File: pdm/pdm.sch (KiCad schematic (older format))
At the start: 46 parts, among them J1 Conn_01x04_Male, J2 Conn_01x06_Female, J3 Conn_01x04_Female, J4 Conn_01x12_Male, M1 Fan, M2 Fan, SW1 SW_Push, U1 SN65HVD233, U2 STM32F042G6Ux, Y1 Crystal_GND24

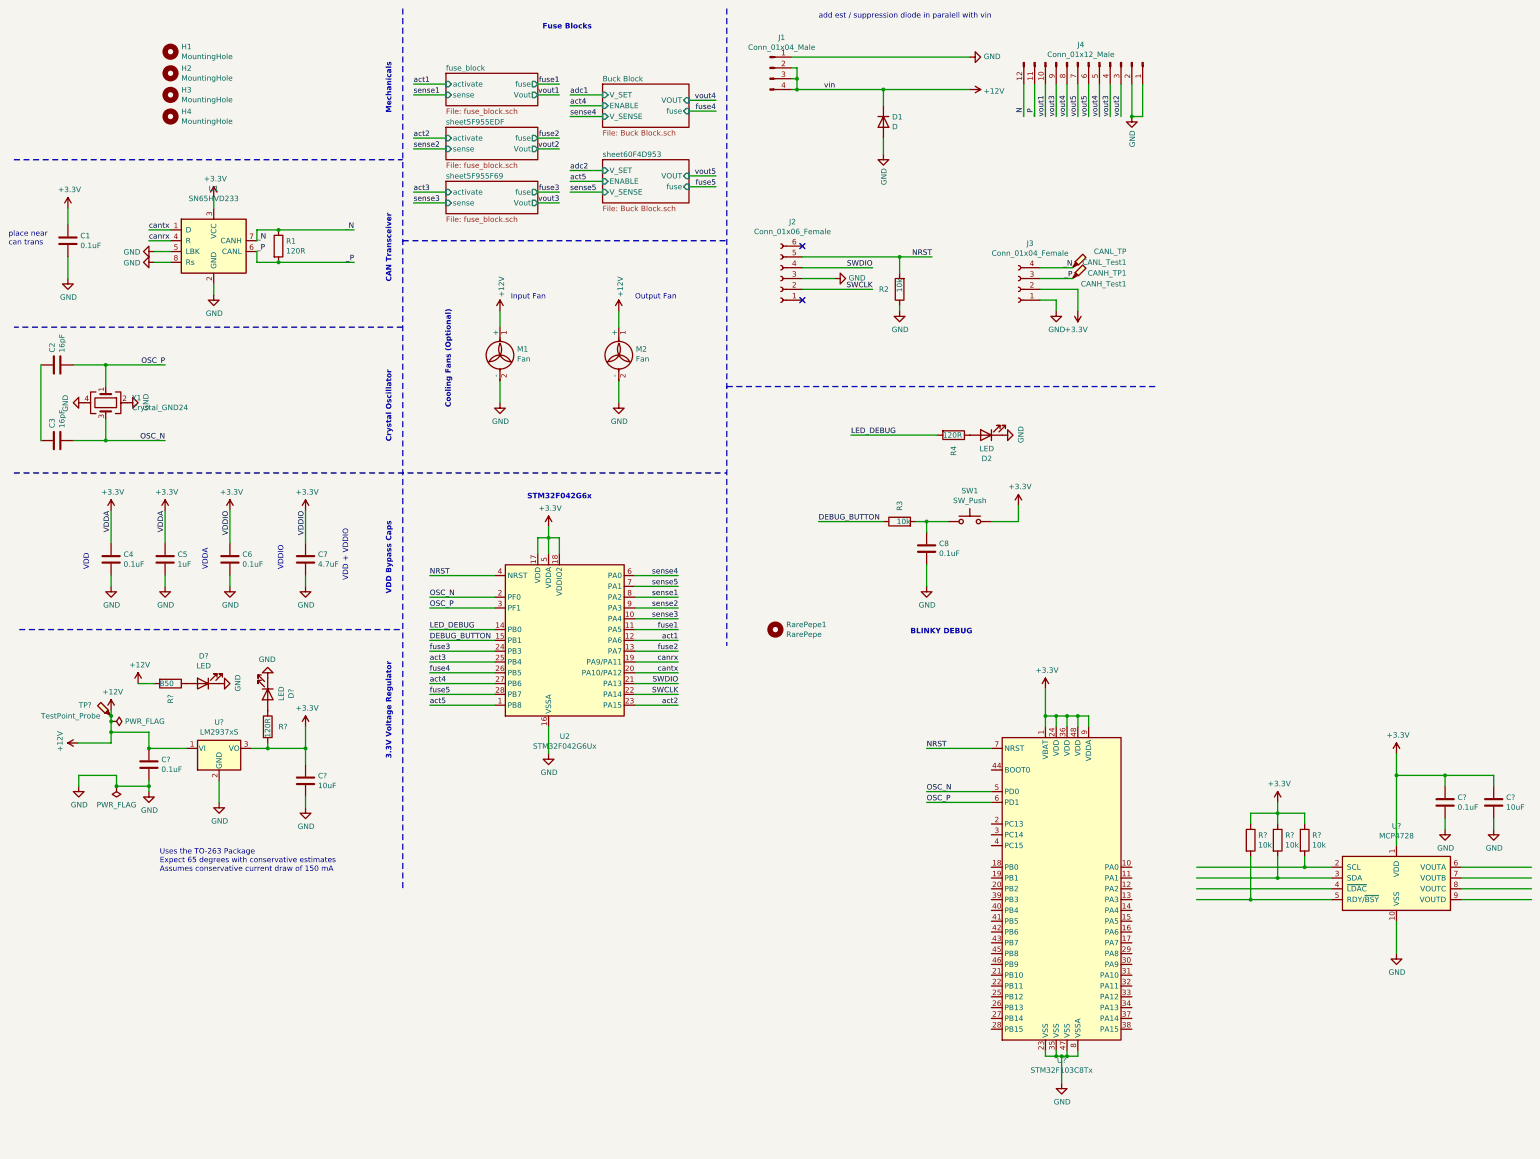
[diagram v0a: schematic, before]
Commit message: fixed schematic
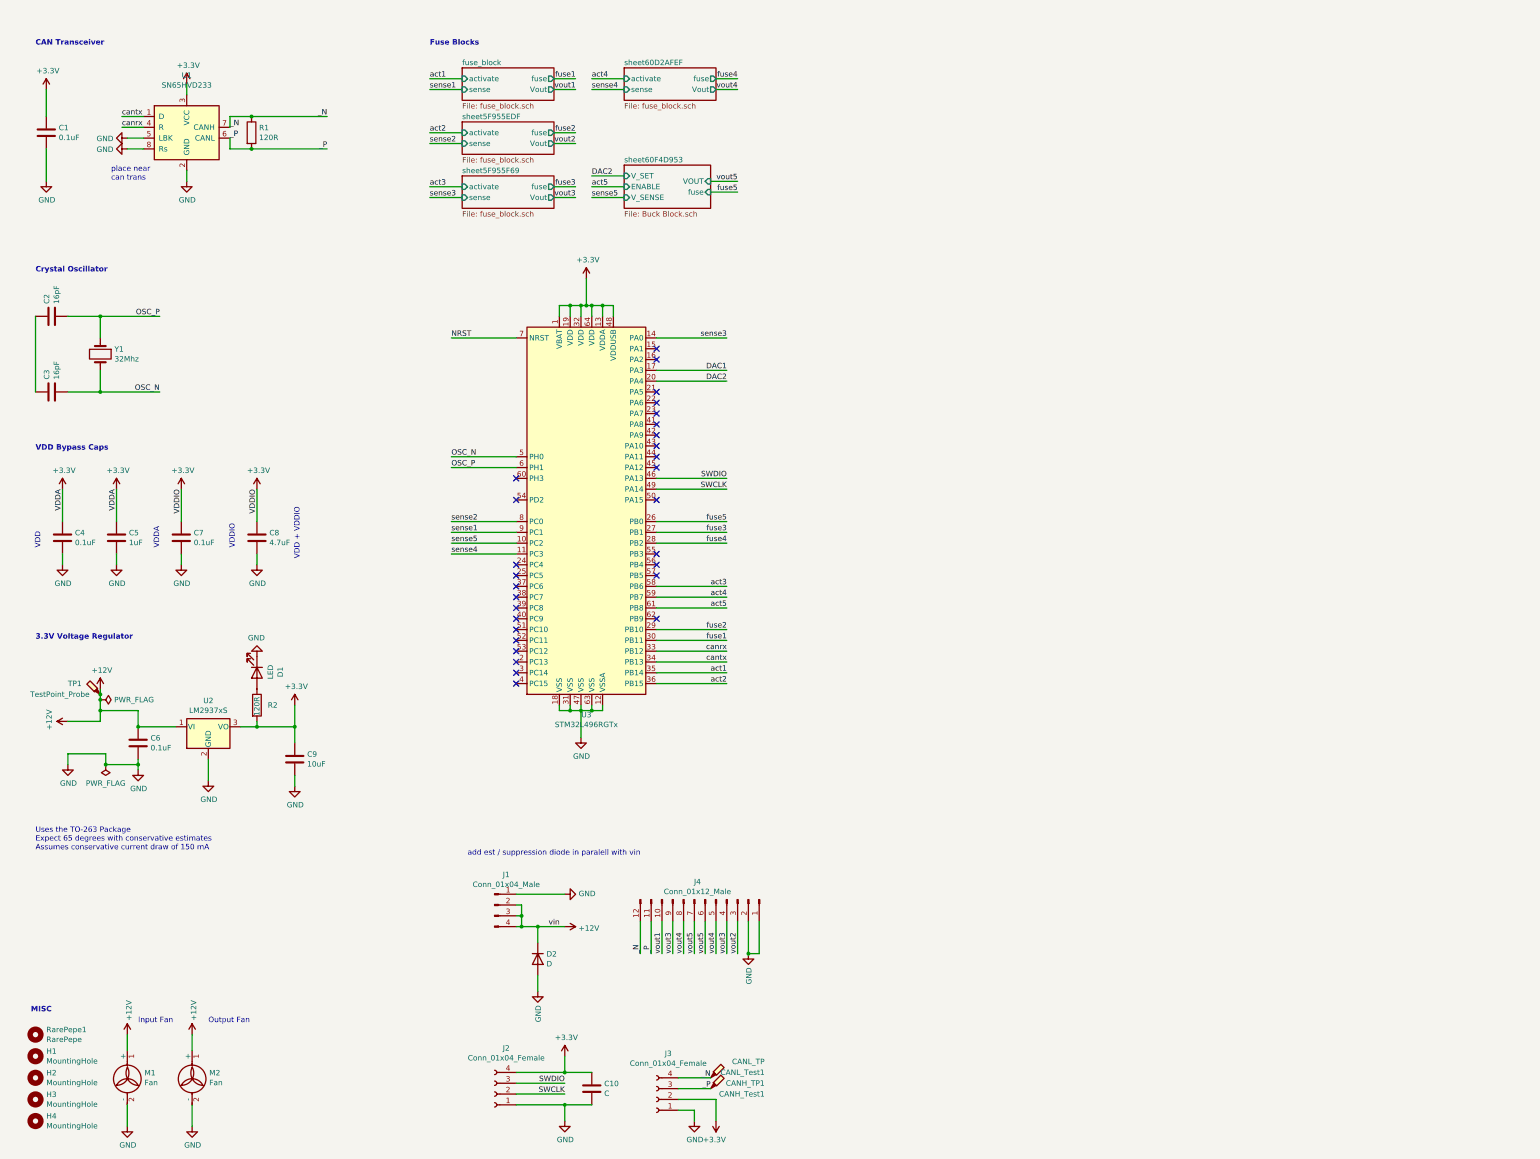
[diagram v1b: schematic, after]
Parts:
- removed C8: 0.1uF, Capacitor_SMD:C_0805_2012Metric_Pad1.18x1.45mm_HandSolder, symbol pdm-rescue:C-Device
- removed C?: 10uF, symbol Device:C
- removed C?: 0.1uF, symbol Device:C
- removed D2, D?: LED, LED_SMD:LED_0805_2012Metric_Pad1.15x1.40mm_HandSolder, symbol pdm-rescue:LED-Device
- removed J2: Conn_01x06_Female, Connector_PinSocket_2.54mm:PinSocket_1x06_P2.54mm_Vertical_SMD_Pin1Left, symbol Connector:Conn_01x06_Female
- removed R2, R3: 10k, Resistor_SMD:R_0805_2012Metric_Pad1.20x1.40mm_HandSolder, symbol pdm-rescue:R-Device
- removed R4: 120R, Resistor_SMD:R_0805_2012Metric_Pad1.20x1.40mm_HandSolder, symbol pdm-rescue:R-Device
- removed R? (x3): 10k, symbol Device:R
- removed R?: 850, Resistor_SMD:R_0805_2012Metric_Pad1.20x1.40mm_HandSolder, symbol pdm-rescue:R-Device
- removed SW1: SW_Push, Button_Switch_THT:SW_PUSH_6mm, symbol pdm-rescue:SW_Push-Switch
- removed U2: STM32F042G6Ux, Package_DFN_QFN:QFN-28_4x4mm_P0.5mm, symbol pdm-rescue:STM32F042G6Ux-MCU_ST_STM32F0
- removed U?: STM32F103C8Tx, Package_QFP:LQFP-48_7x7mm_P0.5mm, symbol MCU_ST_STM32F1:STM32F103C8Tx
- removed U?: MCP4728, Package_SO:MSOP-10_3x3mm_P0.5mm, symbol Analog_DAC:MCP4728
- removed Y1: Crystal_GND24, Crystal:Crystal_SMD_3225-4Pin_3.2x2.5mm_HandSoldering, symbol Device:Crystal_GND24
- added C10: C, Capacitor_SMD:C_0603_1608Metric, symbol Device:C
- added J2: Conn_01x04_Female, Connector_PinHeader_2.54mm:PinHeader_1x04_P2.54mm_Vertical, symbol Connector:Conn_01x04_Female
- added U3: STM32L496RGTx, Package_QFP:LQFP-64_10x10mm_P0.5mm, symbol MCU_ST_STM32L4:STM32L496RGTx
- added Y1: 32Mhz, Crystal:Crystal_SMD_HC49-SD, symbol Device:Crystal
- C1, C2, C3, C4, C5: footprint Capacitor_SMD:C_0805_2012Metric_Pad1.18x1.45mm_HandSolder -> Capacitor_SMD:C_0603_1608Metric
- C6: renamed from C?; footprint Capacitor_SMD:C_0805_2012Metric_Pad1.18x1.45mm_HandSolder -> Capacitor_SMD:C_0603_1608Metric
- C7: renamed from C6; footprint Capacitor_SMD:C_0805_2012Metric_Pad1.18x1.45mm_HandSolder -> Capacitor_SMD:C_0603_1608Metric
- C8: renamed from C7; footprint Capacitor_SMD:C_0805_2012Metric_Pad1.18x1.45mm_HandSolder -> Capacitor_SMD:C_0603_1608Metric
- C9: renamed from C?; footprint (none) -> Capacitor_SMD:C_0603_1608Metric
- gave numbers to parts that had none: 4
- renumbered D1 to D2
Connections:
- net labels added: DAC1, DAC2
- net labels removed: DEBUG_BUTTON, LED_DEBUG, adc1, adc2
- wire segments 203 -> 159
- no-connect marks 2 -> 29
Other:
- note added: "MISC"
- note removed: "BLINKY DEBUG"
- note removed: "Cooling Fans (Optional)"
- note removed: "Mechanicals"
- note removed: "STM32F042G6x"
- moved on the sheet: C1, C2, C3, C4, C5, C6, C7, C8, C9, CANH_TP1, CANL_Test1, D1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
